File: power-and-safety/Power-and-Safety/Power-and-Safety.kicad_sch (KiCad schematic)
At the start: 0 parts

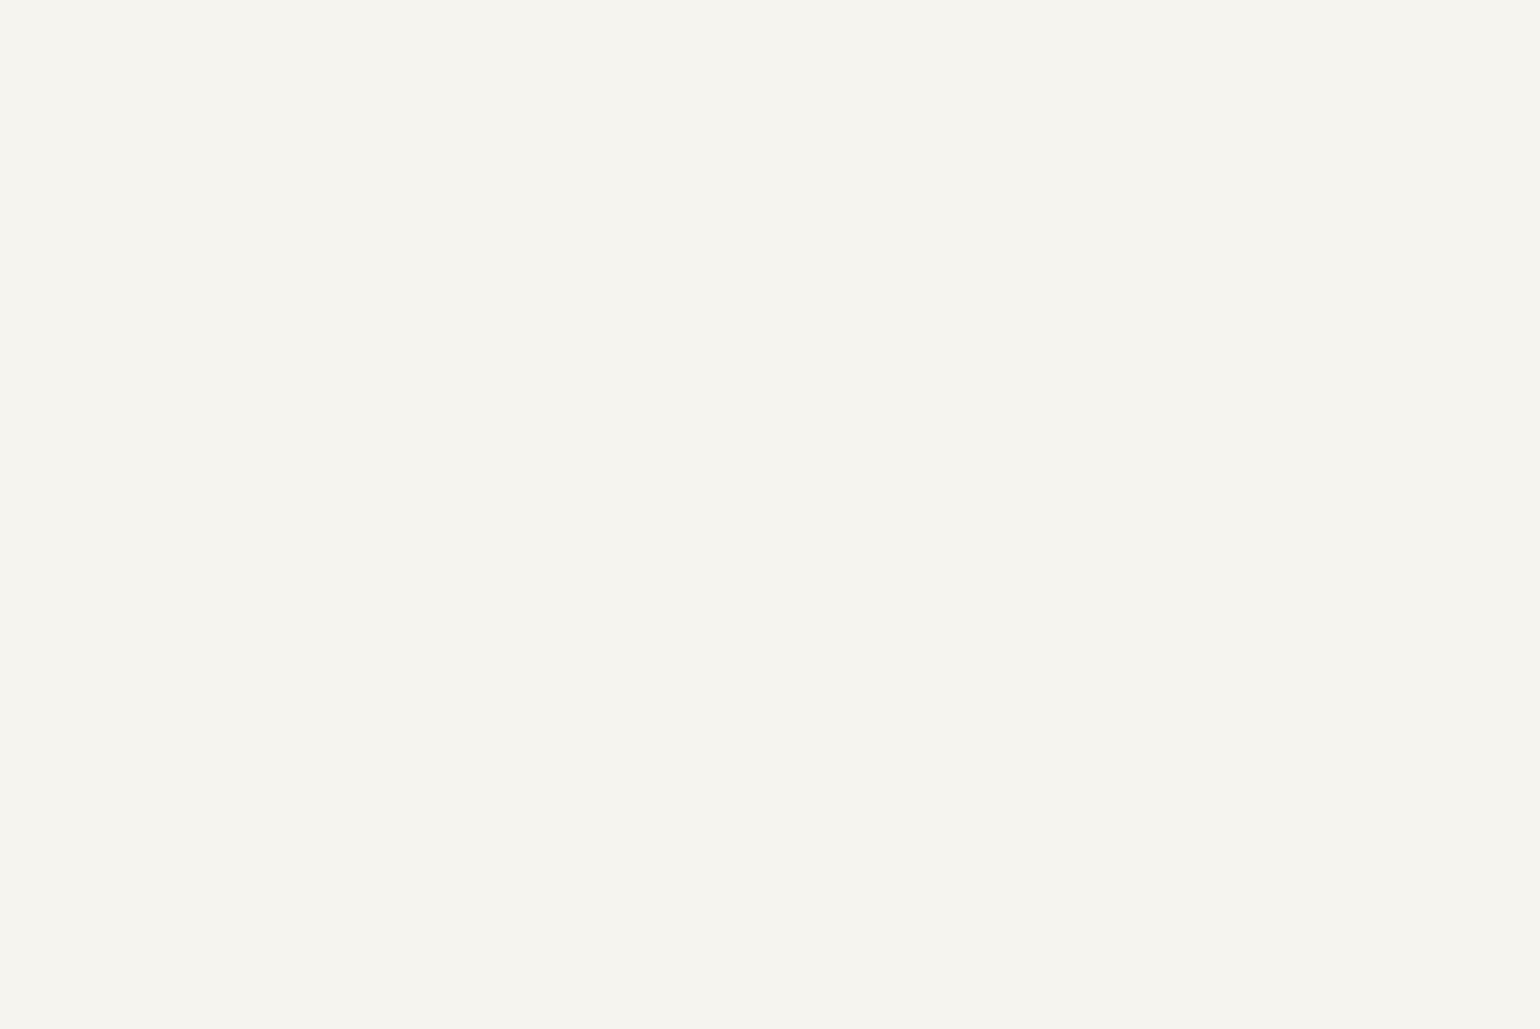
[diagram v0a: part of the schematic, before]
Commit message: worked on emergency power shutoff
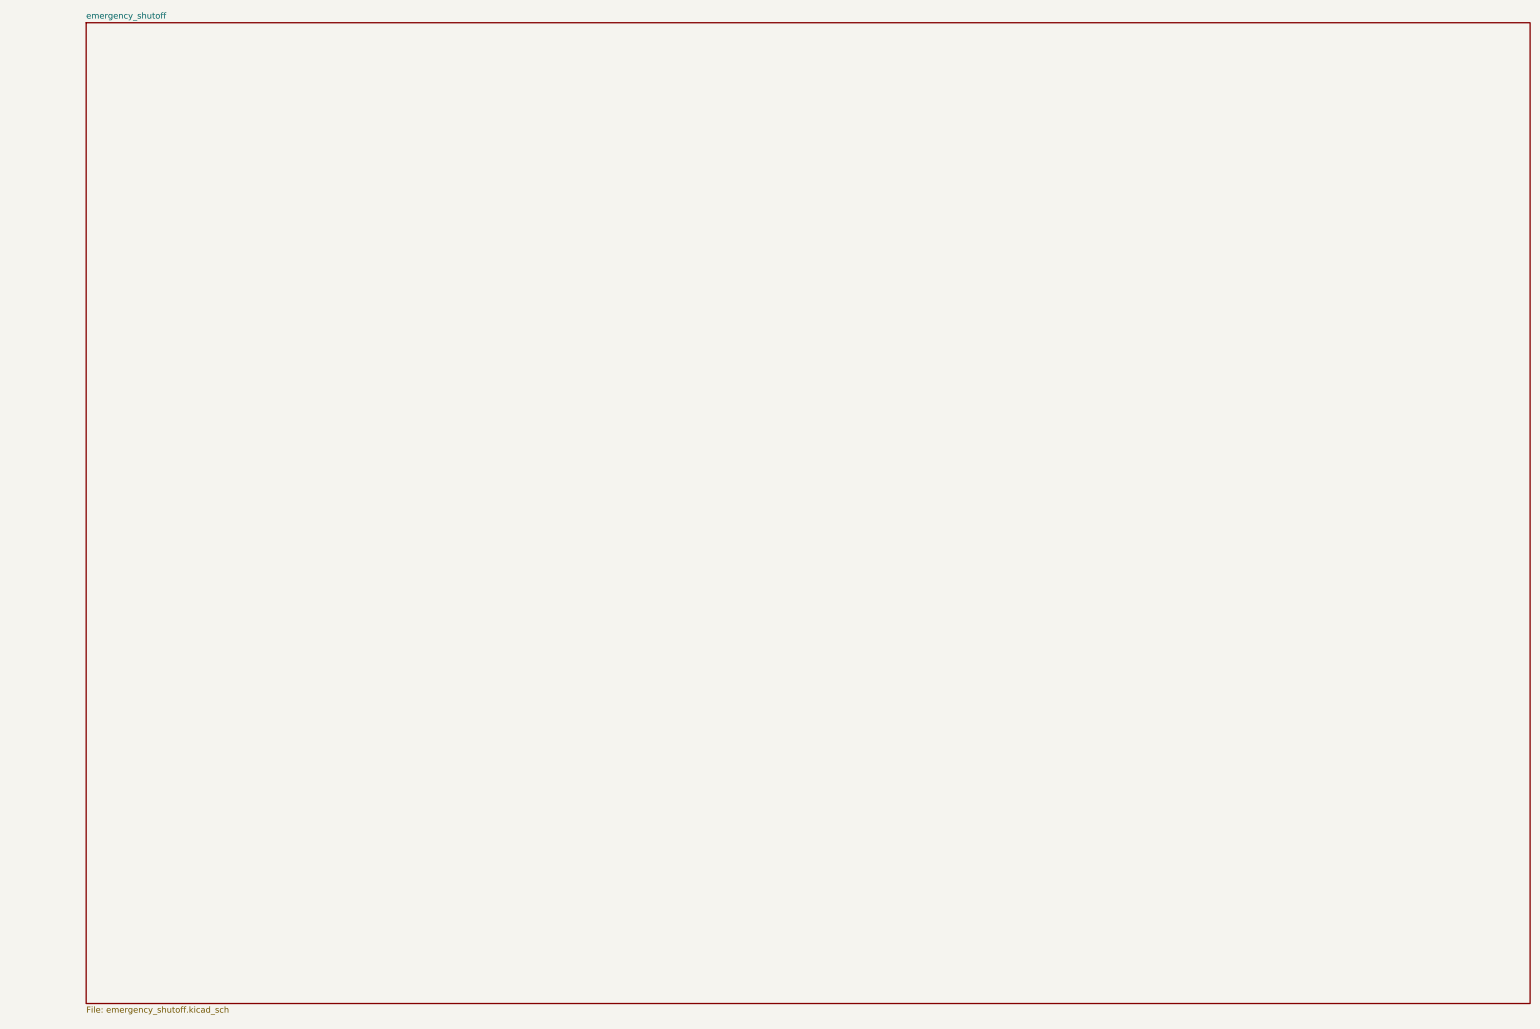
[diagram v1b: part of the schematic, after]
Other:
- added sheet emergency_shutoff (emergency_shutoff.kicad_sch)
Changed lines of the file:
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@@
 	(paper "A4")
+	(sheet
+		(at 631.825 1.27)
+		(size 302.895 205.74)
+		(exclude_from_sim no)
+		(in_bom yes)
+		(on_board yes)
+		(dnp no)
+		(fields_autoplaced yes)
+		(stroke
+			(width 0.1524)
+			(type solid)
+		)
+		(fill
+			(color 0 0 0 0.0000)
+		)
+		(property "Sheetname" "emergency_shutoff"
+			(at 631.825 0.5584 0)
+			(effects
+				(font
+					(size 1.27 1.27)
+				)
+				(justify left bottom)
+			)
+		)
+		(property "Sheetfile" "emergency_shutoff.kicad_sch"
+			(at 631.825 207.5946 0)
+			(effects
+				(font
+					(size 1.27 1.27)
+				)
+				(justify left top)
+			)
+		)
+		(instances
+			(project "Power-and-Safety"
+				(path "/e28a5393-a52f-43fd-ab49-3e8cb48472a2"
+					(page "3")
+				)
+			)
+		)
+	)
 	(sheet
 		(at 323.85 1.27)
